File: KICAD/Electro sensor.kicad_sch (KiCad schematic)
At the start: 3 parts, among them J1 SIM_Card_Shielded, U1 ESP32-WROOM-32D, U2 BC660KGLAA-I03-SNASA

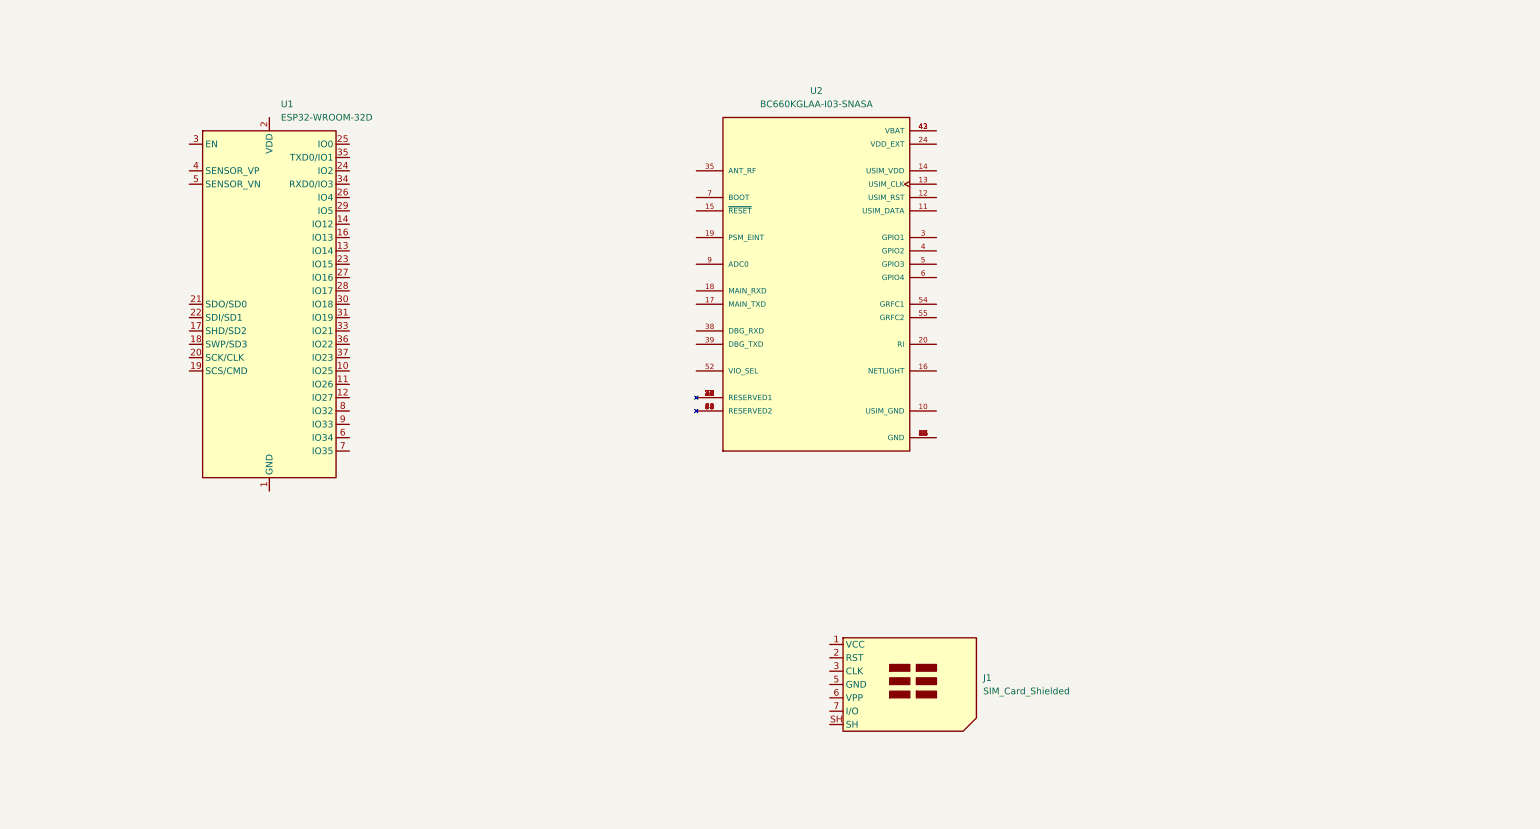
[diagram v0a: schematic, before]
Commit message: update on schematics
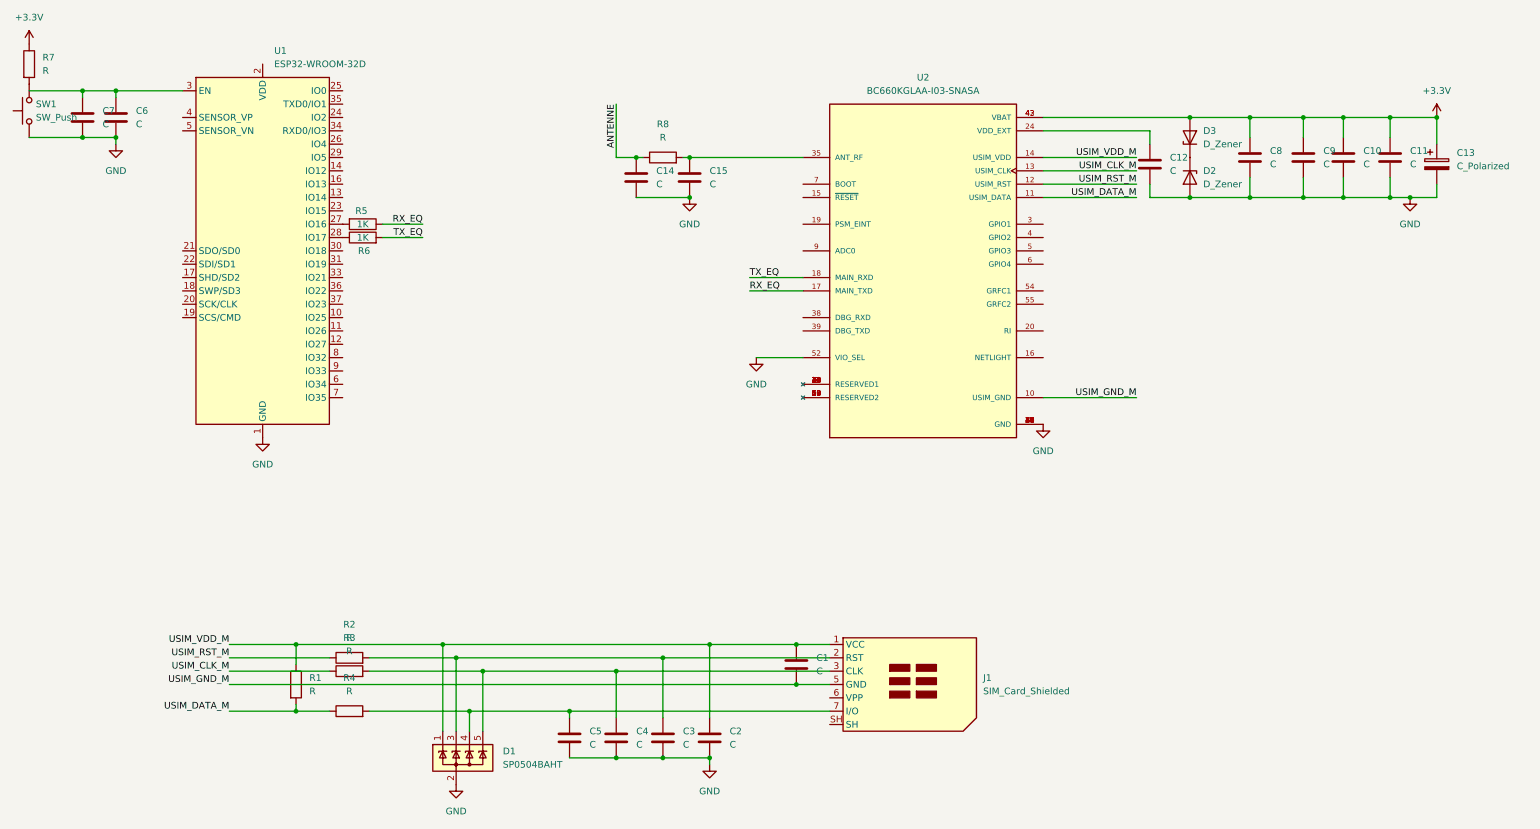
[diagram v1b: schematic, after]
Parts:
- added C1, C10, C11, C12, C14, C15, C2, C3, C4, C5, C6, C7, C8, C9: C, symbol Device:C
- added C13: C_Polarized, symbol Device:C_Polarized
- added D1: SP0504BAHT, Package_TO_SOT_SMD:SOT-23-5, symbol Power_Protection:SP0504BAHT
- added D2, D3: D_Zener, symbol Device:D_Zener
- added R1, R2, R3, R4, R7, R8: R, symbol Device:R
- added R5, R6: 1K, symbol Device:R
- added SW1: SW_Push, symbol Switch:SW_Push
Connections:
- net GND: now reaches U2.1 (GND), U2.27 (GND), U2.34 (GND), U2.36 (GND), U2.37 (GND), U2.40 (GND), U2.41 (GND), U2.56 (GND), U2.57 (GND), U2.58 (GND)
- net GND: now also U1.1 (GND), U1.15 (GND), U1.38 (GND), U1.39 (GND), U2.52 (VIO_SEL), C10.2, C11.2, C12.2, C13.2, C14.2, C15.2, C2.2, C3.2, C4.2, C5.2, C6.2, C7.2, C8.2, C9.2, D1.2 (A), D2.2 (A), SW1.1
- net USIM_GND_M: now reaches U2.10 (USIM_GND)
- net USIM_GND_M: now also J1.5 (GND), C1.2
- net USIM_DATA_M: now reaches U2.11 (USIM_DATA)
- net USIM_DATA_M: now also R1.2, R4.1
- net USIM_RST_M: now reaches U2.12 (USIM_RST)
- net USIM_RST_M: now also R2.1
- net USIM_CLK_M: now reaches U2.13 (USIM_CLK)
- net USIM_CLK_M: now also R3.1
- net USIM_VDD_M: now reaches U2.14 (USIM_VDD)
- net USIM_VDD_M: now also J1.1 (VCC), C1.1, C2.1, D1.1 (K), R1.1
- net RX_EQ: now reaches U2.17 (MAIN_TXD)
- net RX_EQ: now also R5.1
- net TX_EQ: now reaches U2.18 (MAIN_RXD)
- net TX_EQ: now also R6.2
- net at U2.24 (VDD_EXT): now also C12.1
- net at U2.35 (ANT_RF): now also C15.1, R8.2
- net +3.3V: now reaches U2.42 (VBAT), U2.43 (VBAT)
- net +3.3V: now also C10.1, C11.1, C13.1, C8.1, C9.1, D3.2 (A), R7.1
- net at U1.27 (IO16): now also R5.2
- net at U1.28 (IO17): now also R6.1
- net at U1.3 (EN): now also C6.1, C7.1
- net at J1.2 (RST): now also C3.1, D1.3 (K), R2.2
- net at J1.3 (CLK): now also C4.1, D1.5 (K), R3.2
- net at J1.7 (I/O): now also C5.1, D1.4 (K), R4.2
- new net: R7.2, SW1.2
- new net: D2.1 (K), D3.1 (K)
- new net ANTENNE: C14.1, R8.1
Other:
- moved on the sheet: U1, U2
